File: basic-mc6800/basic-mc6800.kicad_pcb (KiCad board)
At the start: 2 copper layers, 100 x 45 mm, 22 parts, among them J1 Conn_01x39_Male, Q1 Q_NMOS_GSD, Q2 Q_NMOS_GSD, U1 74LS137, U2 MC6809, U3 IS61C256AL, U4 28C256, Y1 2-4Mhz

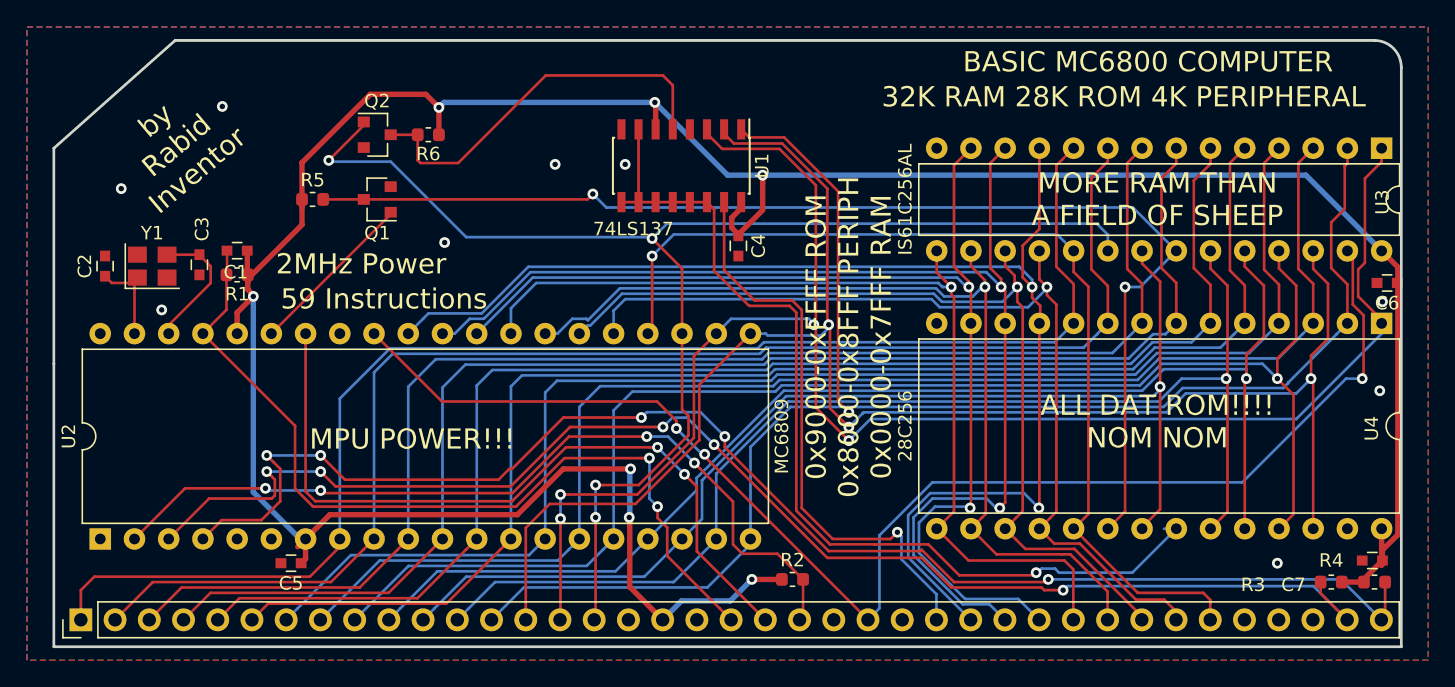
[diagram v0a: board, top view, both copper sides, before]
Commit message: tidied some traces and started io board v1 gerber here
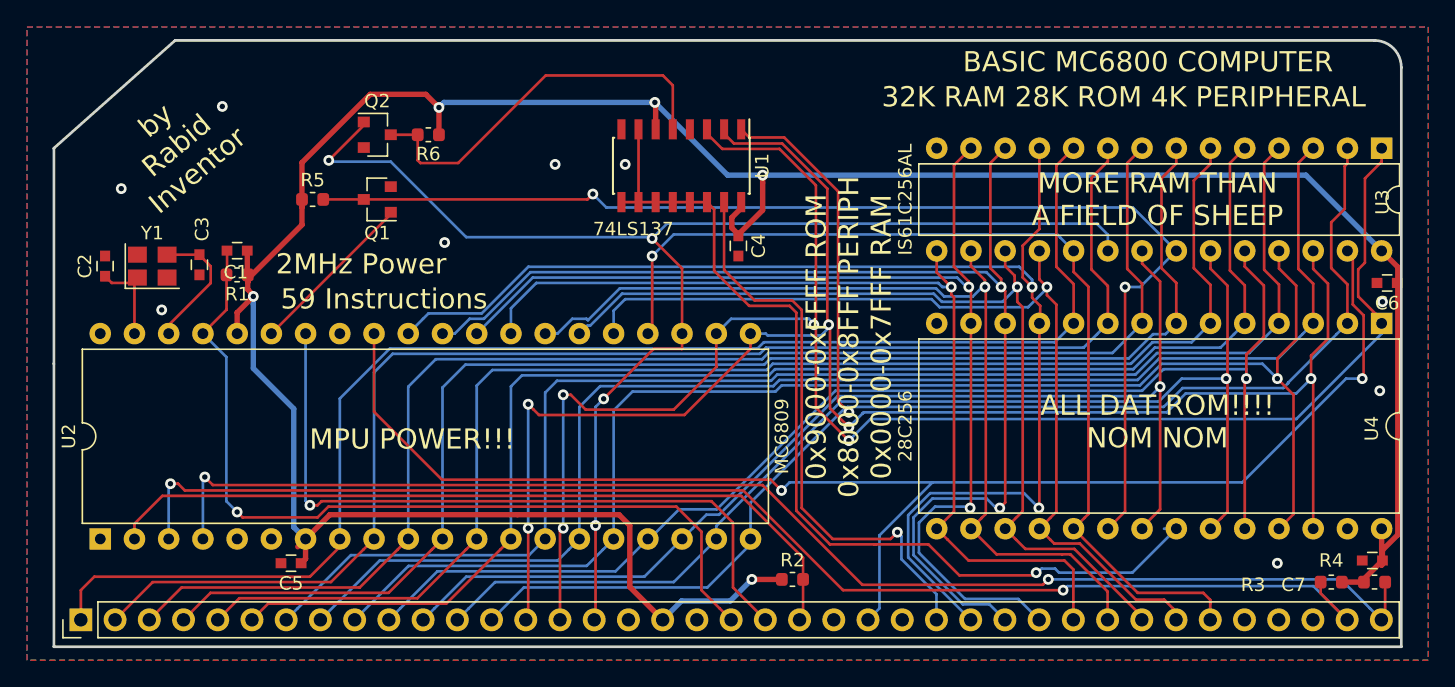
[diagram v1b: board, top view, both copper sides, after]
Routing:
- net /INT3: track 106.3 -> 99.6 mm, vias 5 -> 2
- net +5V: track 219.7 -> 214.1 mm, vias 7 -> 5
- net /INT2: track 104.5 -> 99.8 mm, vias 5 -> 2
- net /INT1: track 62.4 -> 58.2 mm, vias 4 -> 0
- net /A13: track 123.9 -> 128.1 mm, vias 3 -> 5
- net /R_W: track 103.2 -> 107.2 mm, vias 3 -> 2
- net /A14: track 125.6 -> 128.7 mm
- net /E: track 55.9 -> 53.3 mm, vias 2 -> 1
- net /A12: track 117.2 -> 114.8 mm
- net /A11: track 89.0 -> 86.7 mm
- net /A10: track 85.4 -> 83.6 mm
- net /A15: track 100.3 -> 99.3 mm
- net /A9: track 94.4 -> 93.8 mm
- net /RESET: track 64.1 -> 64.4 mm, vias 2 -> 1
